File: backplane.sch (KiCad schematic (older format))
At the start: 37 parts, among them J1 I2C, J2 I2C, J3 SER, J4 PWR, J5 PWR, J6 FAN, J7 PPS, Q4 Q_NMOS_GSD, Q5 Q_PMOS_GSD, SW1 SW_Push, U1 Raspberry_Pi_2_3, U2 IC880A-SPI, U3 DHT22, U4 MP1584_MODULE, U5 MCP3425A0T-E/CH, U6 SHTC3, U7 LM2596_MODULE

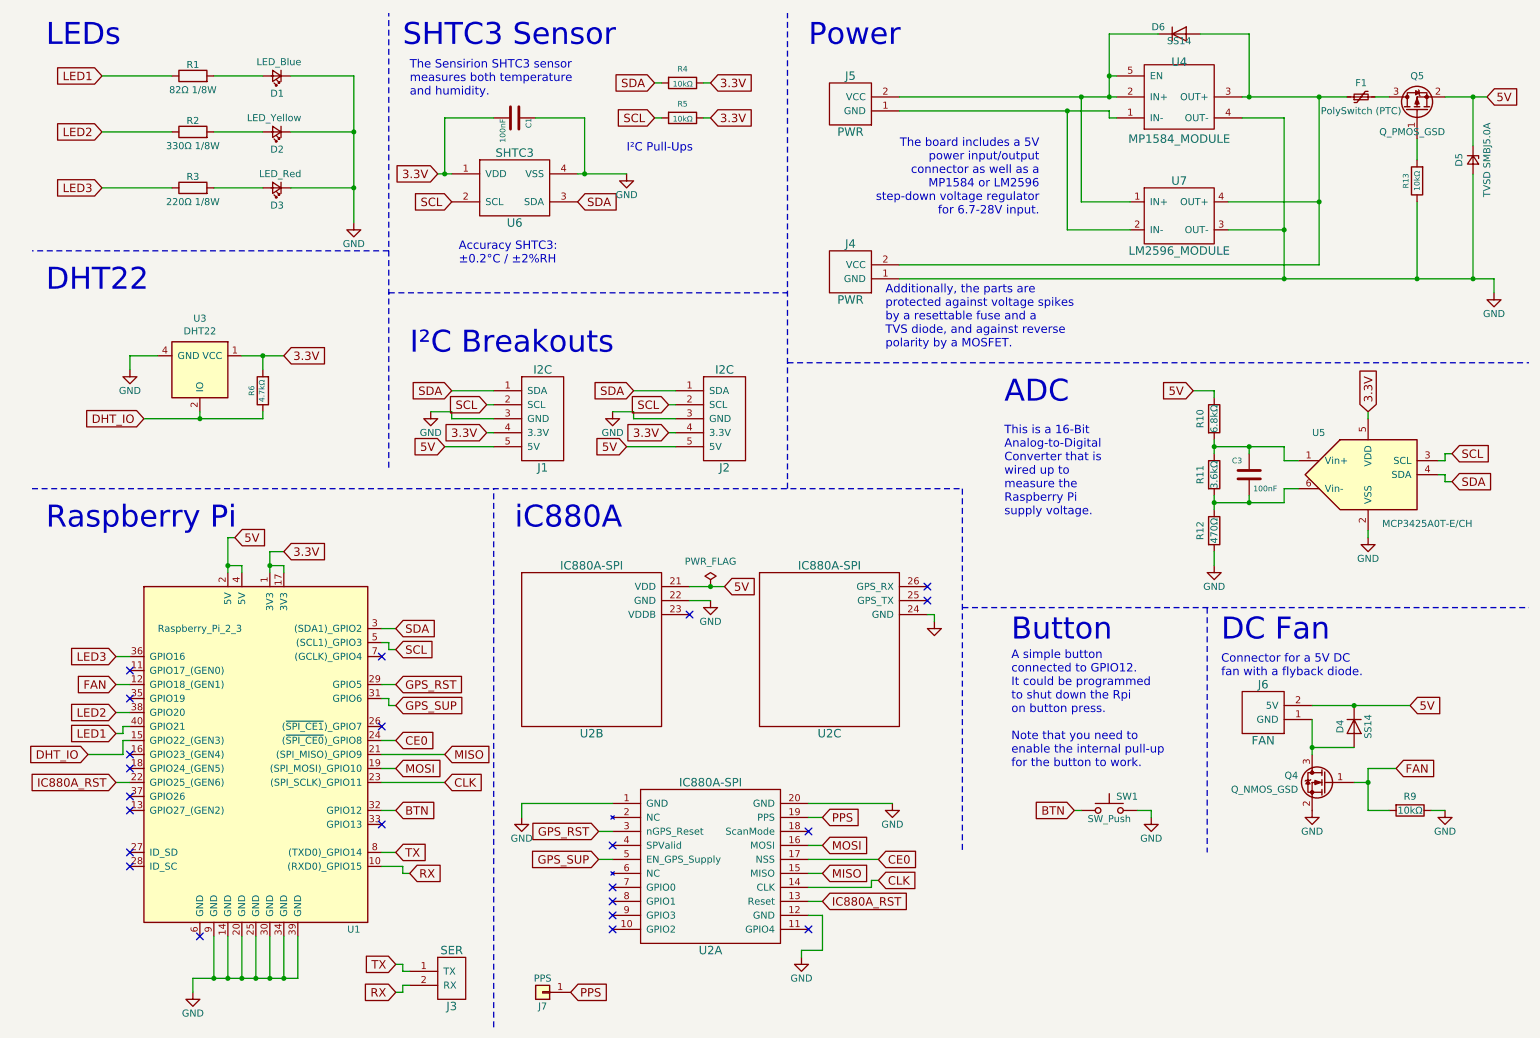
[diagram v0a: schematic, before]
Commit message: added serial link to gps module on ic880a
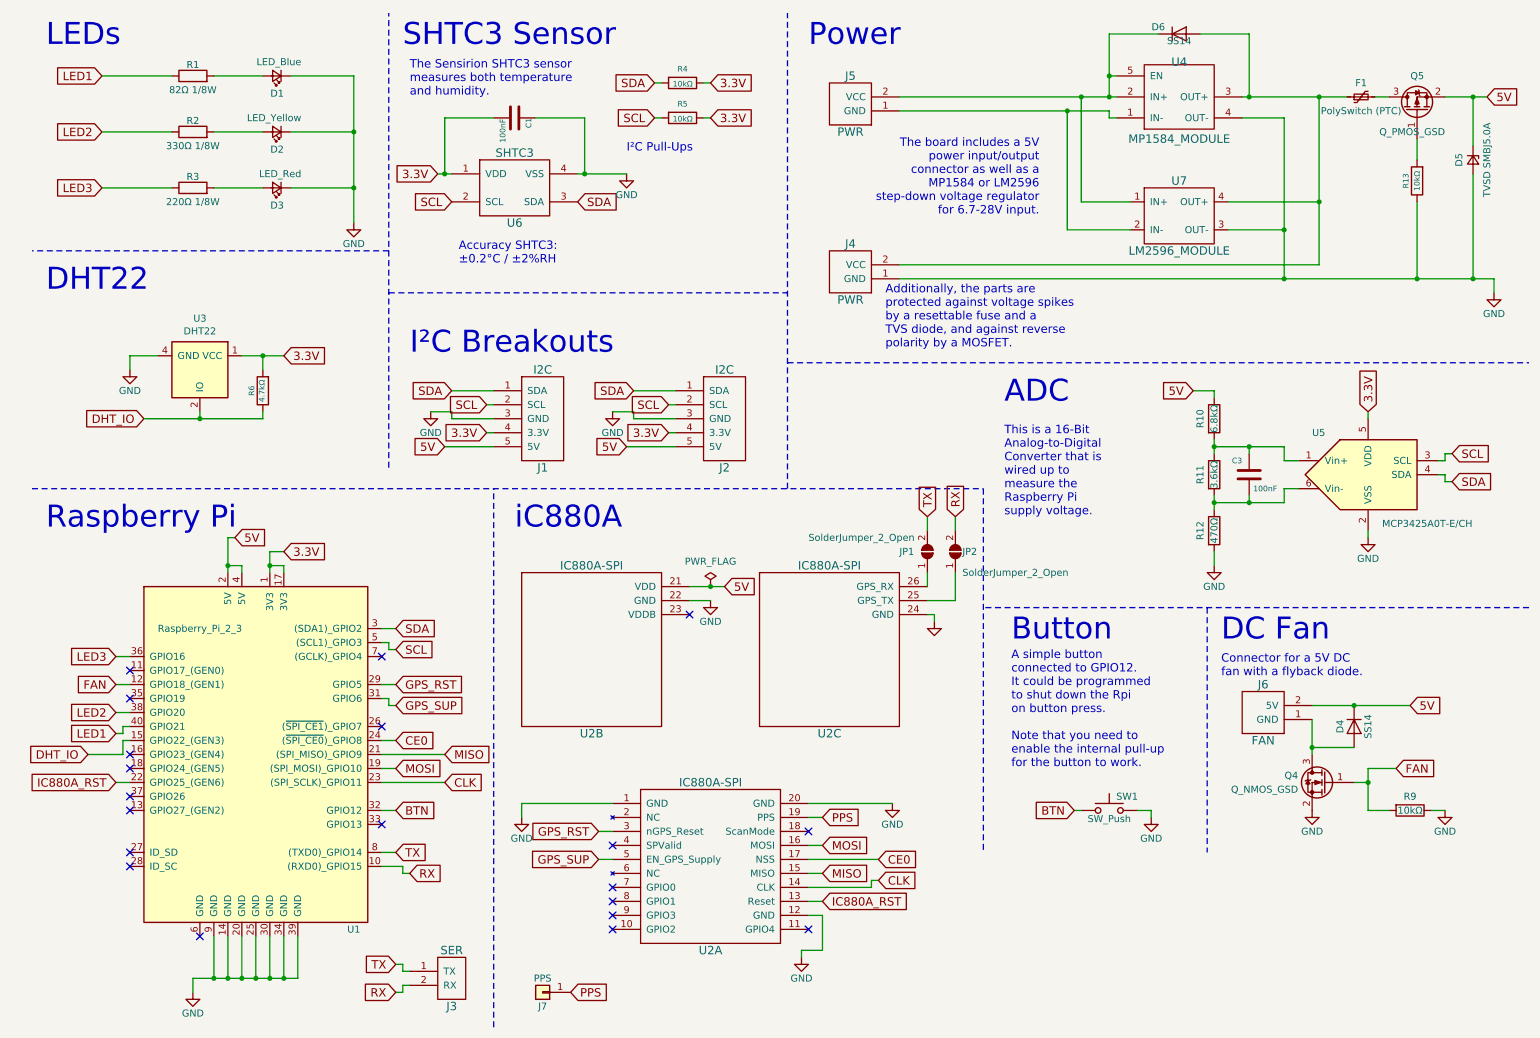
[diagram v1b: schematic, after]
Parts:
- added JP1, JP2: SolderJumper_2_Open, Jumper:SolderJumper-2_P1.3mm_Open_TrianglePad1.0x1.5mm, symbol Jumper:SolderJumper_2_Open
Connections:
- net RX: now also JP2.2 (B)
- net TX: now also JP1.2 (B)
- net at U2.25 (GPS_TX): now also JP2.1 (A)
- net at U2.26 (GPS_RX): now also JP1.1 (A)
- no-connect marks 22 -> 20
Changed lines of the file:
@@
 	1    0    0    -1
 $EndComp
-NoConn ~ 6900 4600
-NoConn ~ 6900 4700
 $Comp
 L backplane-rescue:C-backplane-rescue C1
@@
 	10800 2400 10950 2400
 Wire Notes Line
-	500  3900 7150 3900
-Wire Notes Line
-	7150 3900 7150 6500
-Wire Notes Line
-	7150 4750 11200 4750
-Wire Notes Line
 	5900 3000 11200 3000
 $Comp
@@
 Wire Wire Line
 	9200 650  9200 1100
+Text GLabel 6900 4100 1    60   Input ~ 0
+TX
+Text GLabel 7100 4100 1    60   Input ~ 0
+RX
+Wire Wire Line
+	6900 4600 6900 4500
+Wire Notes Line
+	11200 4750 7300 4750
+Wire Notes Line
+	500  3900 7300 3900
+Wire Notes Line
+	7300 3900 7300 6500
+$Comp
+L Jumper:SolderJumper_2_Open JP1
+U 1 1 5DAE6269
+P 6900 4350
+F 0 "JP1" V 6900 4550 50  0000 R CNN
+F 1 "SolderJumper_2_Open" V 7000 5200 50  0000 R CNN
+F 2 "Jumper:SolderJumper-2_P1.3mm_Open_TrianglePad1.0x1.5mm" H 6900 4350 50  0001 C CNN
+F 3 "~" H 6900 4350 50  0001 C CNN
+	1    6900 4350
+	0    -1   -1   0
+$EndComp
+$Comp
+L Jumper:SolderJumper_2_Open JP2
+U 1 1 5DAE719B
+P 7100 4350
+F 0 "JP2" V 7100 4300 50  0000 R CNN
+F 1 "SolderJumper_2_Open" V 6950 4300 50  0000 R CNN
+F 2 "Jumper:SolderJumper-2_P1.3mm_Open_TrianglePad1.0x1.5mm" H 7100 4350 50  0001 C CNN
+F 3 "~" H 7100 4350 50  0001 C CNN
+	1    7100 4350
+	0    -1   -1   0
+$EndComp
+Wire Wire Line
+	6900 4100 6900 4200
+Wire Wire Line
+	7100 4100 7100 4200
+Wire Wire Line
+	7100 4500 7100 4700
+Wire Wire Line
+	6900 4700 7100 4700
 $EndSCHEMATC
